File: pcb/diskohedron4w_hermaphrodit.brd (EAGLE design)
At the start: 88.5 x 57.3 mm, 20 parts, among them X1 87758-1216, X2 87758-1216

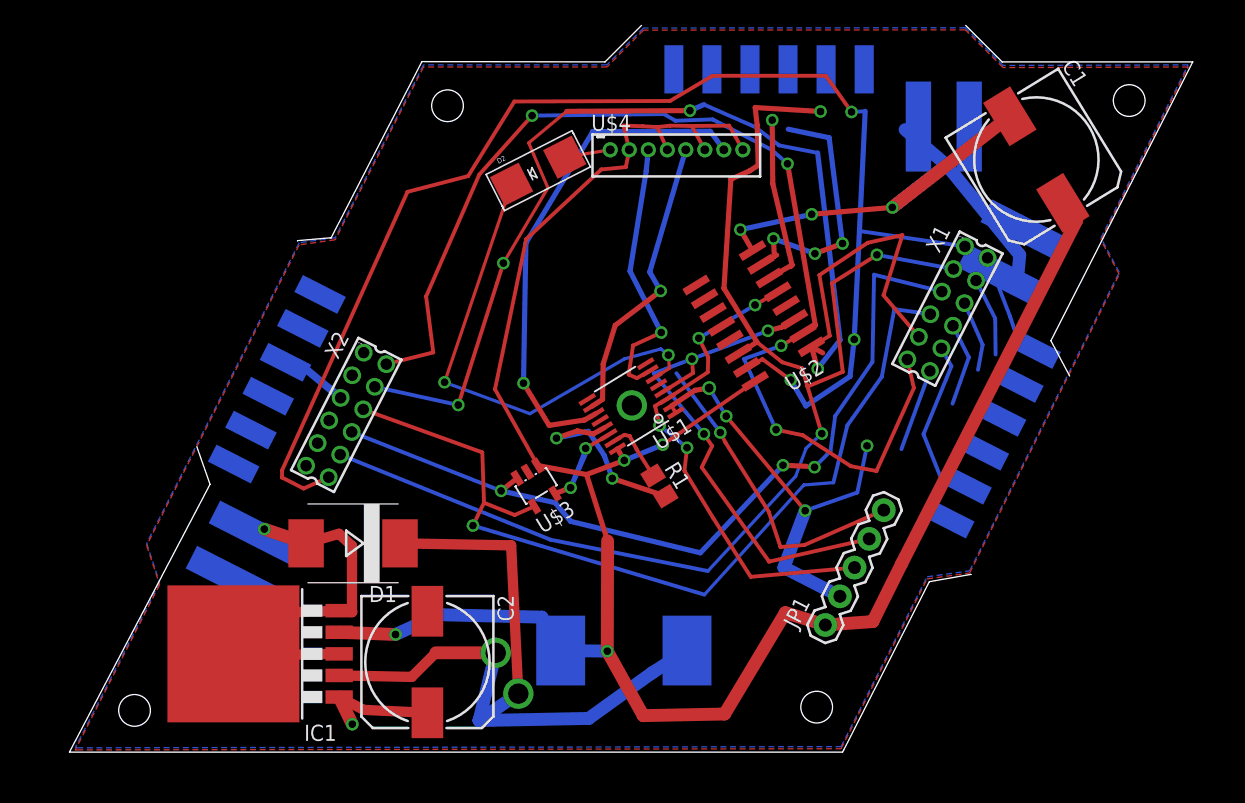
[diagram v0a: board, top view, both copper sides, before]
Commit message: first pcb freeze
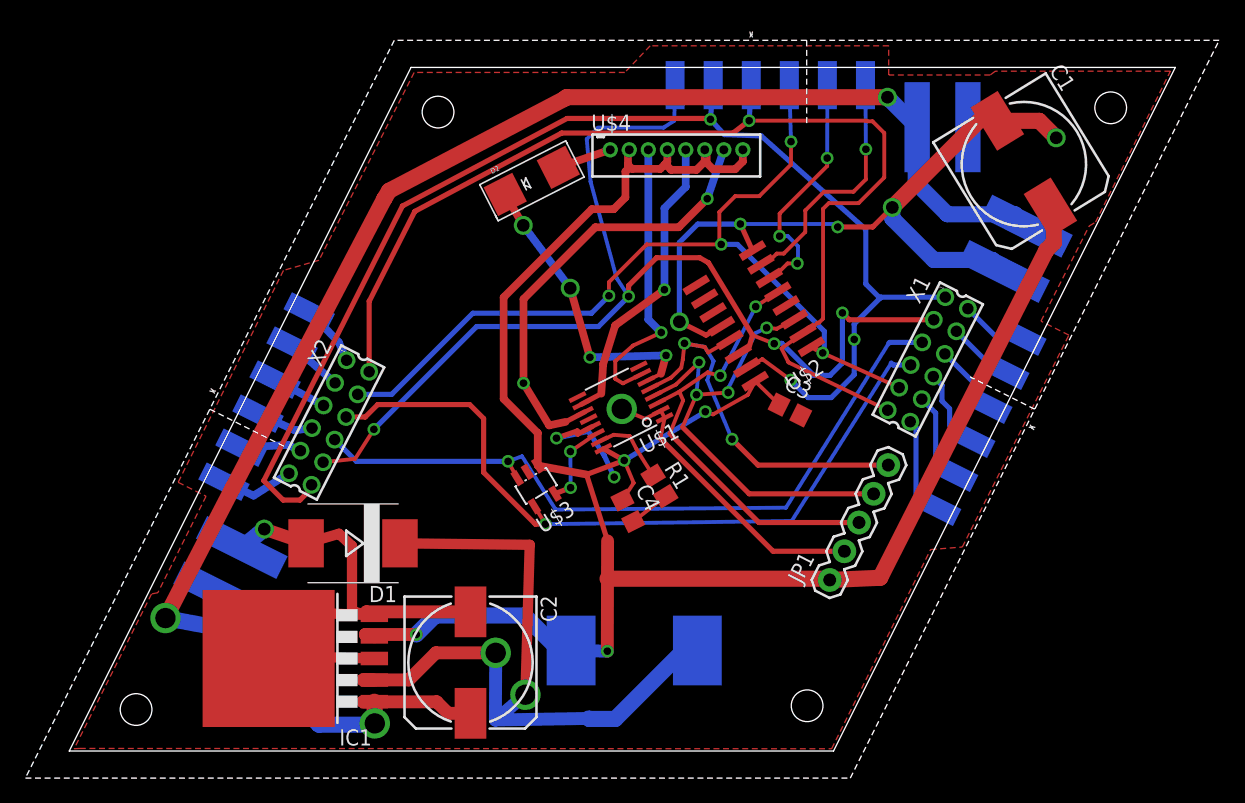
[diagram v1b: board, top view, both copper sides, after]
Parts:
- added C3, C4: (no value), rcl:C0805
- moved X1 4.29 mm to (67.7, 30.9)
- moved JP1 3.57 mm to (60.0, 13.5)
- moved C2 3.40 mm to (31.6, 6.99)
- moved IC1 2.80 mm to (18.3, 7.31)
- moved U$11 1.59 mm to (21.1, 35.8), turned to 296.6 degrees
- moved U$12 1.54 mm to (17.1, 16.4), turned to 296.6 degrees
- moved X2 1.48 mm to (20.5, 25.9)
- moved U$5 1.40 mm to (66.1, 18.1), turned to 116.6 degrees
- moved U$8 1.25 mm to (64.8, 51.1)
- moved C1 1.05 mm to (75.3, 46.3)
- moved D2 0.94 mm to (36.5, 45.0)
- moved U$1 0.83 mm to (43.5, 27.1), turned to 116.6 degrees
- moved L1 0.82 mm to (44.5, 7.94)
- moved U$6 0.36 mm to (70.2, 37.4), turned to 116.6 degrees
- moved U$7 0.11 mm to (72.7, 46.2)
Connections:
- net +3V3: now also C3.1, C4.1
- net GND: now also C3.2, C4.2, U$2.12
- net OE-: now also U$8.P$5
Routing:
- net +24V: track 9.58 -> 131.2 mm, vias 1 -> 3
- net CLK-: track 97.6 -> 70.7 mm
- net GND: track 126.6 -> 143.7 mm, vias 11 -> 9
- net N$3: track 38.4 -> 23.5 mm, vias 2 -> 4
- net OE+: track 102.1 -> 89.8 mm, vias 3 -> 4
- net DATAOUT+: track 70.9 -> 59.9 mm
- net OE-: track 110.3 -> 102.1 mm
- net +3V3: track 170.2 -> 162.9 mm
- net DATAOUT-: track 65.2 -> 58.1 mm, vias 3 -> 1
- net OE: track 24.8 -> 31.8 mm, vias 1 -> 2
- net OE-L: track 0.00 -> 5.87 mm
- net DATA+: track 13.8 -> 19.3 mm, vias 1 -> 3
- net CLK+L: track 0.00 -> 4.91 mm
- net OE+L: track 0.00 -> 4.79 mm
- net LED3: track 40.1 -> 35.4 mm, vias 1 -> 2
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- removed copper zone on layer 16, net GND
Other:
- board size 88.5 x 57.3 mm -> 94.1 x 58.1 mm
- board text added: "rotation angles: 63.4 26.6"

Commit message: rev. a almost fixed, first gerber-cam process
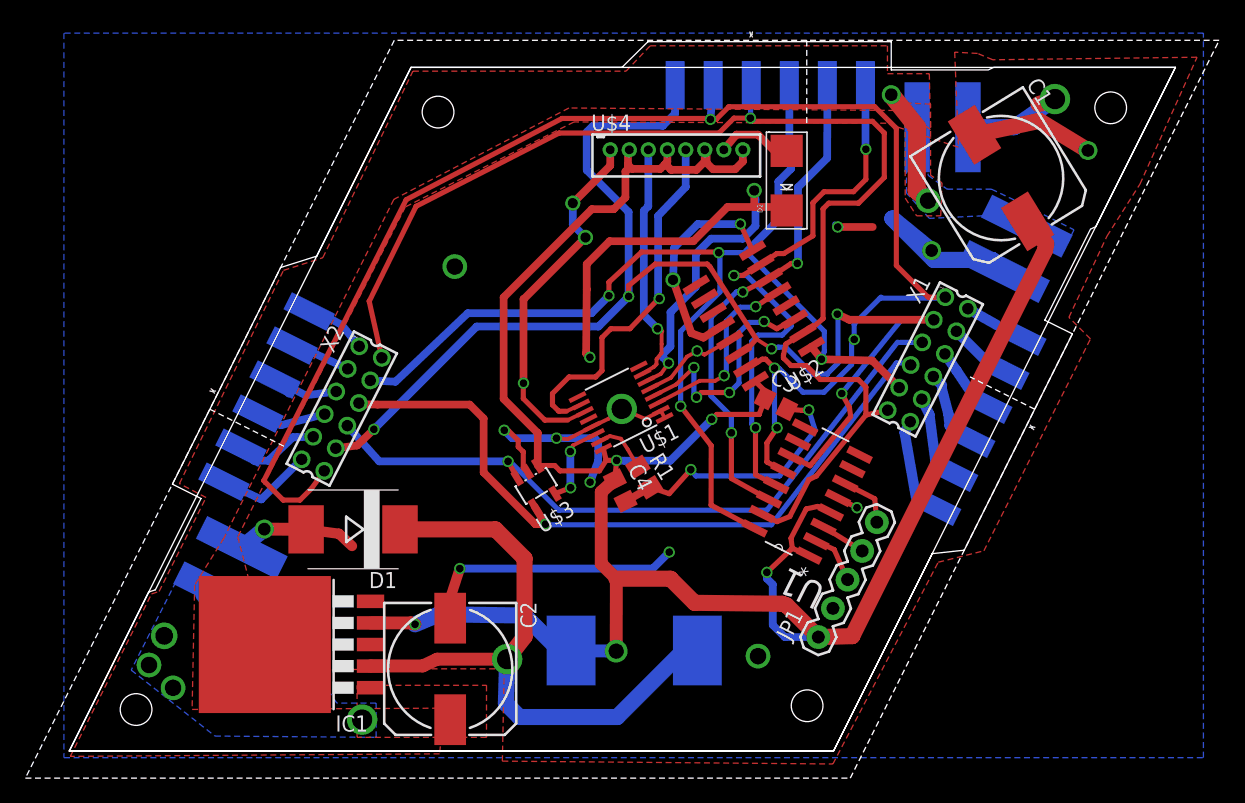
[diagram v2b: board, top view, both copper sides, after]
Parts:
- added U1: SN65LVDS047D, Texas Instruments_By_element14_Batch_1:SOIC127P600X175-16N
- moved D2 20.1 mm to (56.6, 45.0), turned to 90 degrees
- moved JP1 4.59 mm to (59.1, 9.00)
- moved C1 2.11 mm to (73.5, 45.2)
- moved C4 1.71 mm to (43.4, 20.6)
- moved C2 1.68 mm to (30.0, 6.49)
- moved X2 1.49 mm to (21.5, 27.0)
- moved R1 1.39 mm to (45.3, 21.6)
- moved C3 1.21 mm to (55.7, 27.4)
- moved IC1 1.14 mm to (18.0, 8.41)
- moved D1 1.10 mm to (22.4, 17.5)
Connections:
- new net EXTCLK: JP1.4, U1.3
- new net EXTDATA: JP1.3, U1.2
- new net EXTOE: JP1.5, U1.6
- net +3V3: now also U1.1, U1.4
- net CLK: no longer JP1.4
- net CLK+: now also U1.15
- net CLK-: now also U1.16
- net DATA+: now also U1.14
- net DATA-: now also U1.13
- net DATA-IN: no longer JP1.3
- net GND: now also U1.5
- net LED0: now also U$4.7; no longer U$4.1
- net LED3: now also U$4.1; no longer U$4.7
- net OE: no longer JP1.5
- net OE+: now also U1.11
- net OE-: now also U1.12
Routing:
- net +24V: track 131.2 -> 11.3 mm, vias 3 -> 6
- net DATA-: track 19.5 -> 44.6 mm, vias 1 -> 3
- net OE: track 31.8 -> 7.83 mm, vias 2 -> 1
- net +3V3: track 162.9 -> 186.8 mm, vias 4 -> 5
- net N$3: track 23.5 -> 47.1 mm, vias 4 -> 3
- net CLK-: track 70.7 -> 94.2 mm
- net DATA+: track 19.3 -> 40.3 mm
- net OE-: track 102.1 -> 122.5 mm, vias 3 -> 4
- net DATA-IN: track 35.3 -> 15.1 mm
- net CLK: track 38.1 -> 19.2 mm
- net OE+: track 89.8 -> 106.9 mm, vias 4 -> 5
- net CLK+: track 87.6 -> 101.5 mm
- net N$2: track 60.8 -> 51.3 mm, vias 2 -> 1
- net LED3: track 35.4 -> 29.0 mm, vias 2 -> 3
- net LED2: track 23.8 -> 29.2 mm
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- added copper zone on layer 1, net +24V
- added copper zone on layer 16, net +24V
- added copper zone on layer 16, net GND
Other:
- outline, holes or cut-outs redrawn
